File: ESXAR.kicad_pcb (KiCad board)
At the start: 2 copper layers, 71.1 x 58.7 mm, 46 parts, among them P1 ANALOG, P10 USB_A, P11 USB_B, P12 SERVO/INPUT, P13 ANALOG, P16 BREADBOARD_POWER, P17 SENSOR, P18 EXTIO, P19 UNIVERSAL, P2 BREADBOARD, P20 UNIVERSAL, P3 PROGRAM, P4 OPAMP EX, P5 MODEJP, P6 VCCJP, P7 GNDJP, P8 SCREW, SW1 RESET, U1 ESP-WROOM-02, U2 NJM4556A, U3 AUDIO_JACK, U5 TLP222A, U6 Mini360

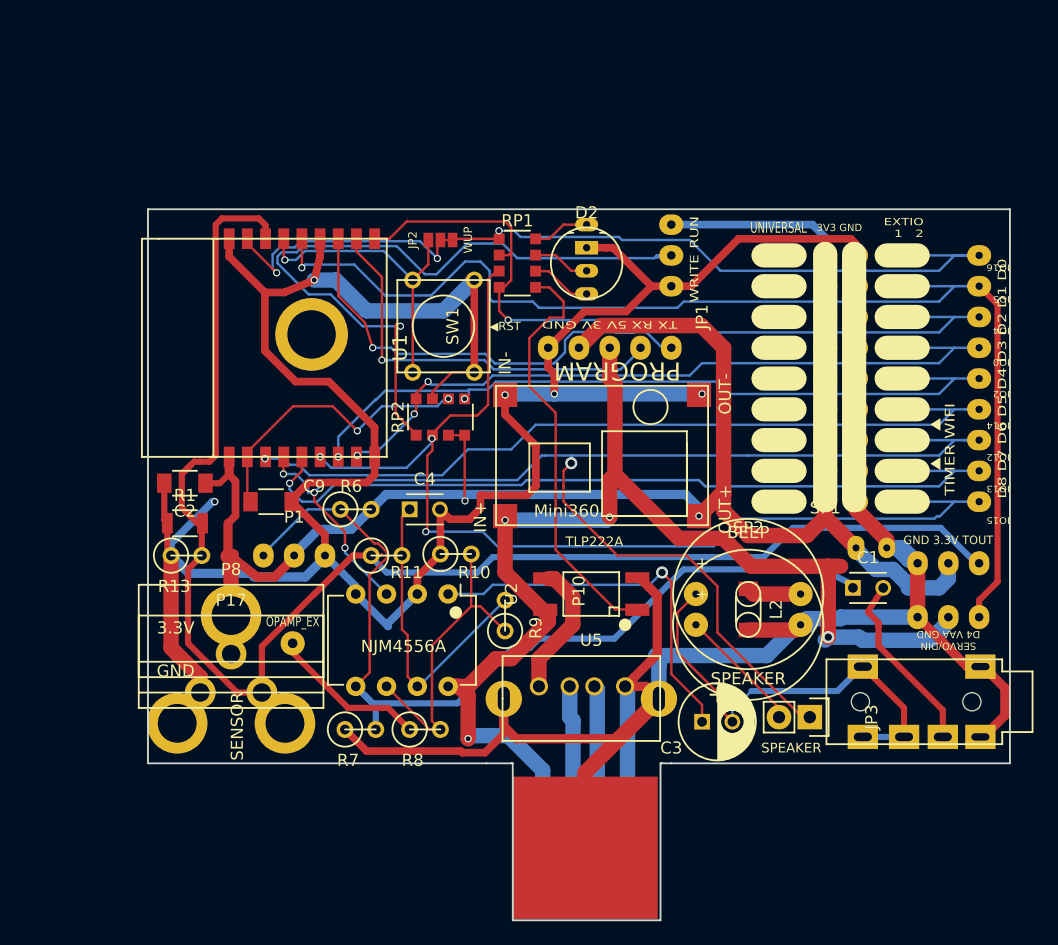
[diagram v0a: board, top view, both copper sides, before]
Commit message: Ver 20160804 Layout Change.
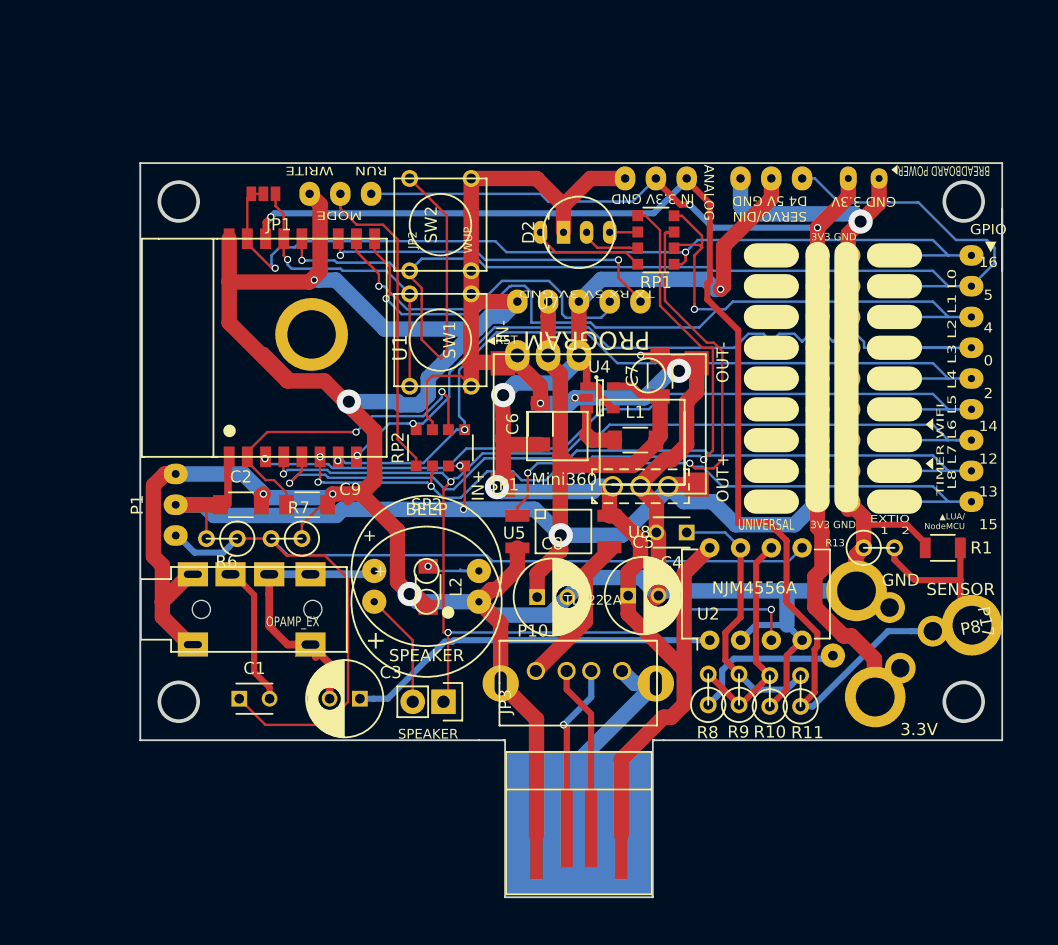
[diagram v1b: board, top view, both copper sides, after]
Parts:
- added C5: 100uF, Capacitors_ThroughHole:C_Radial_D6.3_L11.2_P2.5, F.Cu at (176.8, 125.9)
- added C6: 10uF, library:C_1206_HandSoldering_Small, F.Cu at (169.5, 111.7)
- added C7: 10uF, library:C_1206_HandSoldering_Small, F.Cu at (179.4, 107.7)
- added C8: 100uF, Capacitors_ThroughHole:C_Radial_D6.3_L11.2_P2.5, F.Cu at (169.3, 126.0)
- added L1: 4.7uH, library:C_1206_HandSoldering_Small, F.Cu at (177.4, 113.0)
- added SW2: DIN, Buttons_Switches_ThroughHole:SW_PUSH_SMALL, F.Cu at (161.3, 95.2)
- added U4: MT5201-3.3N, TO_SOT_Packages_SMD:SOT-23-5, F.Cu at (174.5, 109.5)
- added U7: LD1117CV33, Power_Integrations:TO-220, F.Cu at (170.2, 106.0)
- added U8: TA48M033F, TO_SOT_Packages_THT:SOT126_SOT32_Housing_Vertical_Mirrored, F.Cu at (177.8, 116.8)
- P11: moved to F.Cu
- moved U3 69.0 mm to (139.1, 127.0), turned to 0 degrees
- moved R1 62.6 mm to (202.7, 121.9)
- moved P8 59.9 mm to (203.9, 128.5), turned to 280 degrees
- moved P17 57.3 mm to (201.3, 128.9), turned to 280 degrees
- moved R13 57.2 mm to (197.5, 121.9)
- moved C1 51.5 mm to (144.7, 134.4)
- moved P4 44.6 mm to (193.7, 130.8)
- moved P13 39.9 mm to (179.1, 91.4)
- moved P12 39.0 mm to (188.6, 91.4)
- moved R11 35.9 mm to (191.0, 133.7), turned to 90 degrees
- moved P16 30.5 mm to (196.2, 91.4)
- moved JP3 30.3 mm to (161.5, 134.6)
- moved C3 28.3 mm to (154.6, 134.4), turned to 180 degrees
- moved R10 28.3 mm to (188.5, 133.7), turned to 90 degrees
- moved JP1 27.8 mm to (153.0, 92.7), turned to 0 degrees
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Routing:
- net +3V3: track 162.5 -> 217.9 mm, vias 3 -> 6
- net GND: track 372.5 -> 416.7 mm, vias 5 -> 10
- net Net-(JP1-Pad2): track 60.0 -> 26.3 mm, vias 1 -> 0
- net Net-(P13-Pad1): track 138.5 -> 121.3 mm, vias 0 -> 1
- net Net-(C3-Pad2): track 37.1 -> 23.6 mm
- net Net-(P12-Pad1): track 98.4 -> 111.5 mm
- net Net-(P18-Pad3): track 67.1 -> 79.1 mm, vias 1 -> 2
- net Net-(P3-Pad1): track 37.5 -> 29.0 mm, vias 1 -> 2
- net Net-(RP1-Pad5): track 35.1 -> 43.0 mm, vias 0 -> 2
- net Net-(R10-Pad2): track 25.7 -> 18.7 mm
- net Net-(P3-Pad2): track 33.8 -> 28.4 mm
- net +5V: track 104.4 -> 109.7 mm, vias 4 -> 3
- net Net-(D2-Pad1): track 4.70 -> 9.35 mm
- net Net-(P18-Pad5): track 64.0 -> 68.6 mm
- net Net-(L1-Pad1): track 0.00 -> 4.59 mm
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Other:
- board size 71.1 x 58.7 mm -> 71.1 x 60.6 mm
- board text added: "ANALOG"
- board text added: "BREADBOARD POWER▶"
- board text added: "ESXAR Ver.20160804"
- board text added: "GND 3.3V"
- board text added: "GPIO ▼ 16 5 4 0 2 14 12 13 15"
- board text added: "IN 3.3V GND"
- board text added: "IO16 IO5 IO4 IO0 IO2 IO14 IO12 IO13 IO15"
- board text added: "L8 L7 L6 L5 L4 L3 L2 L1 L0"
- board text added: "MODE"
- board text added: "SERVO/DIN D4 5V GND"
- board text added: "▲LUA/ NodeMCU"
- board text removed: "D0:IO16 D1:IO5 D2:IO4 D3:IO0 D4:IO2 D5:IO14 D6:IO12 D7:IO13 D8:IO15 D9:RX D10:TX"
- board text removed: "D8 D7 D6 D5 D4 D3 D2 D1 D0"
- board text removed: "ESXAR Ver.20160802"
- board text removed: "GND 3.3V TOUT"
- board text removed: "IO15 IO13 IO12 IO14 IO2 IO0 IO4 IO5 IO16"
- board text removed: "SERVO/DIN D4 VAA GND"

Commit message: Ver.20160805 change outline, rayout, delete opamp, etc...
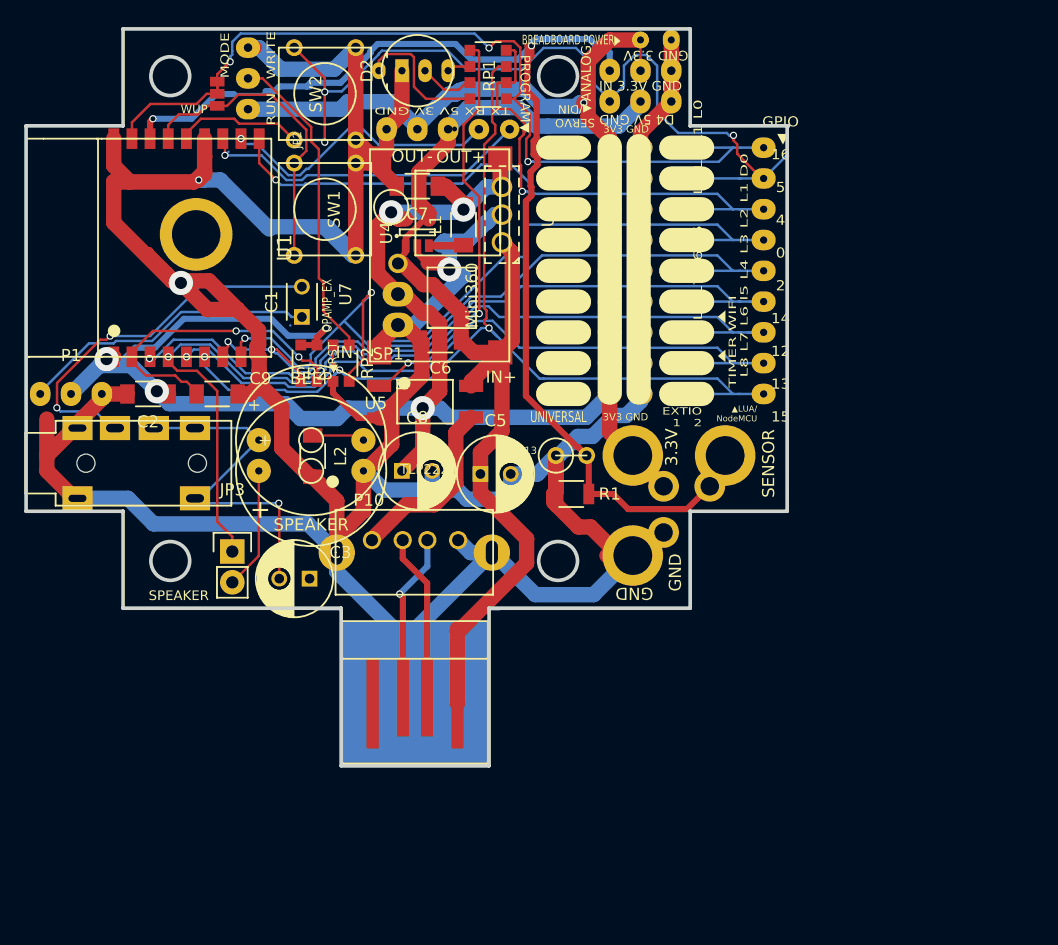
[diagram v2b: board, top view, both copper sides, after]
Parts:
- removed C4: 0.1uF, Capacitors_ThroughHole:C_Disc_D3_P2.5
- removed P4: OPAMP EX, Wire_Pads:SolderWirePad_single_0-8mmDrill
- removed R10, R11, R6, R7, R8, R9: 4.7kΩ, Discret:R1
- removed U2: NJM4556A, Housings_DIP:DIP-8_W7.62mm
- JP1, P17, P8: moved to B.Cu
- moved OSHW 35.6 mm to (132.1, 97.2)
- moved C1 31.9 mm to (149.9, 102.9), turned to 90 degrees
- moved R1 31.0 mm to (172.1, 117.5)
- moved R13 26.5 mm to (172.1, 114.3)
- moved C7 25.4 mm to (159.4, 92.1), turned to 180 degrees
- moved U8 25.2 mm to (166.4, 94.4), turned to 270 degrees
- moved L1 22.7 mm to (163.2, 95.2), turned to 90 degrees
- moved P8 21.8 mm to (184.8, 118.1), turned to 90 degrees
- moved JP3 21.4 mm to (144.1, 122.2), turned to 0 degrees
- moved P17 21.3 mm to (182.2, 119.4), turned to 90 degrees
- moved P16 20.6 mm to (179.1, 80.0)
- moved U4 20.3 mm to (159.4, 95.9), turned to 90 degrees
- moved RP1 19.4 mm to (165.2, 82.9)
- moved P18 19.3 mm to (182.9, 99.1)
- moved P20 19.3 mm to (172.7, 99.1)
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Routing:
- net Net-(C1-Pad1): track 82.6 -> 24.6 mm
- net GND: track 416.7 -> 365.0 mm, vias 10 -> 3
- net Net-(JP3-Pad1): track 117.6 -> 81.2 mm, vias 4 -> 1
- net Net-(C3-Pad1): track 30.9 -> 0.00 mm
- net Net-(P12-Pad1): track 111.5 -> 85.3 mm, vias 1 -> 3
- net +3V3: track 217.9 -> 194.9 mm, vias 6 -> 7
- net Net-(C4-Pad1): track 22.5 -> 0.00 mm
- net Net-(P13-Pad1): track 121.3 -> 101.8 mm, vias 1 -> 2
- net Net-(C1-Pad2): track 11.7 -> 31.0 mm, vias 0 -> 2
- net Net-(R10-Pad2): track 18.7 -> 0.00 mm
- net +5V: track 109.7 -> 92.3 mm, vias 3 -> 1
- net Net-(P4-Pad1): track 13.2 -> 0.00 mm
- net Net-(P18-Pad3): track 79.1 -> 69.1 mm
- net Net-(RP1-Pad5): track 43.0 -> 34.4 mm
- net Net-(P18-Pad8): track 67.4 -> 58.9 mm
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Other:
- board size 71.1 x 60.6 mm -> 62.9 x 60.9 mm
- board text added: "D4 5V GND"
- board text added: "ESXAR Ver.20160805"
- board text added: "L8 L7 L6 l5 L4 L3 L2 L1 D0"
- board text added: "PROGRAM▼"
- board text added: "SERVO ◀/DIN"
- board text removed: "ESXAR Ver.20160804"
- board text removed: "PROGRAM"
- board text removed: "SERVO/DIN D4 5V GND"
